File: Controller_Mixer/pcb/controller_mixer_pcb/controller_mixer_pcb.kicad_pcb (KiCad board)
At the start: 2 copper layers, 144.8 x 104.1 mm, 31 parts, among them J1 Conn_01x08_Male, J10 Conn_01x08_Male, J15 Conn_01x05_Male, J16 Conn_01x05_Male, J19 Conn_01x08_Male, J2 Conn_01x08_Male, J20 Conn_01x08_Male, J3 Conn_01x08_Male, J4 Conn_01x08_Male, J5 Conn_01x05_Male, J6 Conn_01x05_Male, J7 Conn_01x08_Male, J8 Conn_01x08_Male, J9 Conn_01x08_Male, U3 Teensy4.1

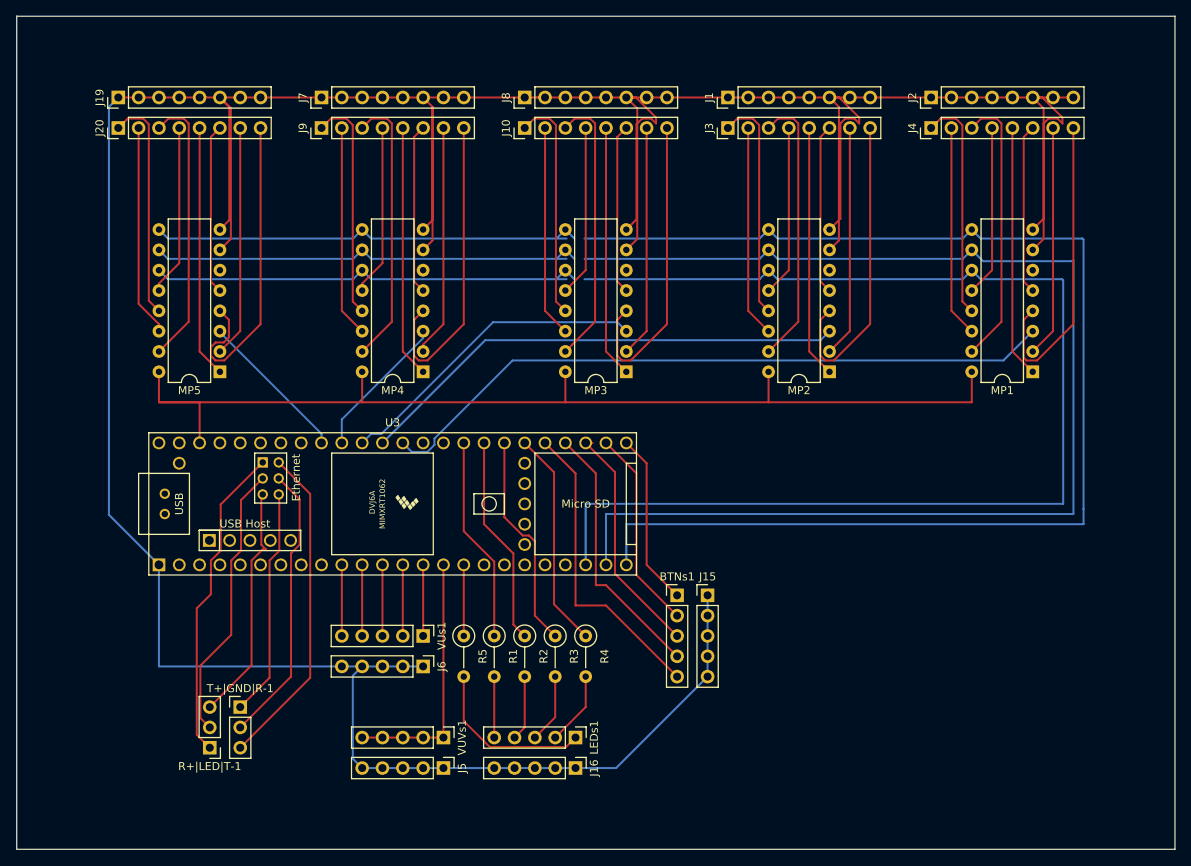
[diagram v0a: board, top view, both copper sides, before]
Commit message: daily edits
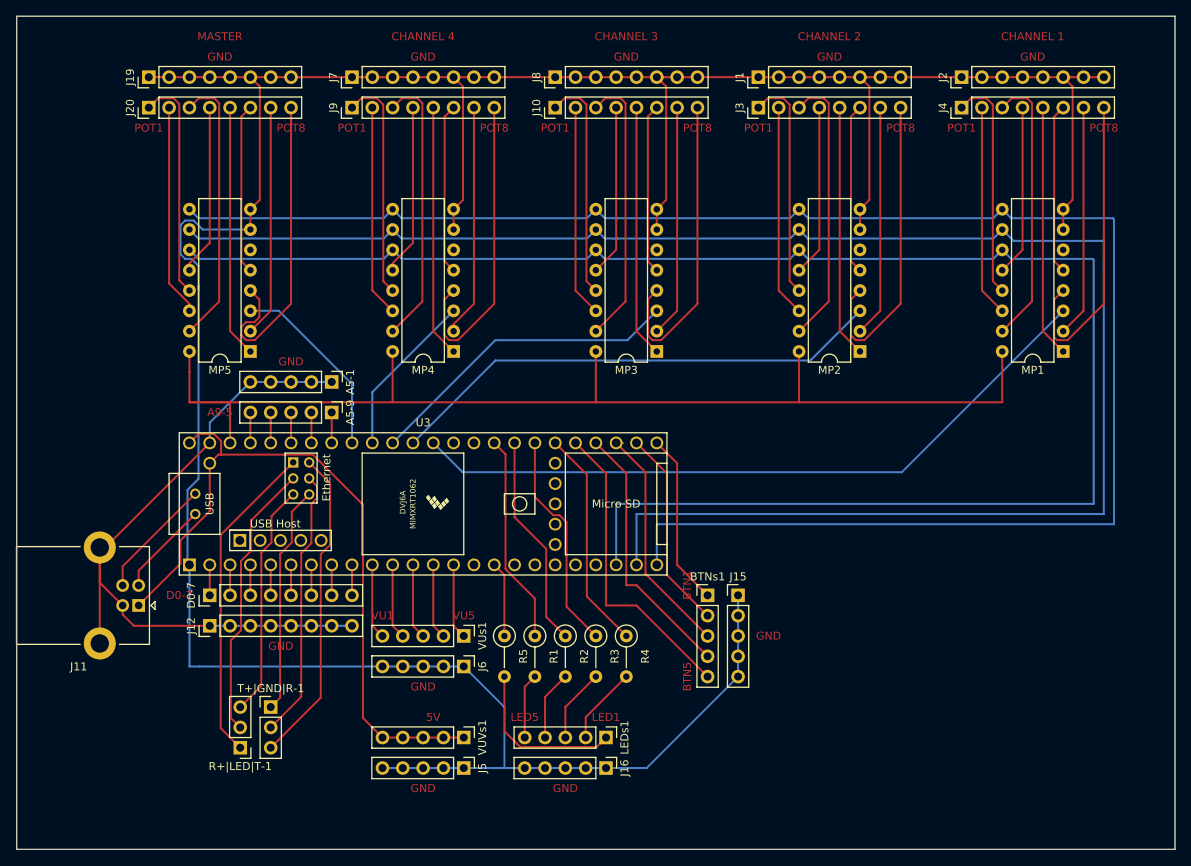
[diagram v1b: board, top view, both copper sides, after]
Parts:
- added A5-1: Conn_01x05_Male, Connector_PinHeader_2.54mm:PinHeader_1x05_P2.54mm_Vertical, F.Cu at (97.8, 85.1)
- added A5-9: Conn_01x05_Male, Connector_PinHeader_2.54mm:PinHeader_1x05_P2.54mm_Vertical, F.Cu at (97.8, 88.9)
- added D0-7: Conn_01x08_Male, Connector_PinHeader_2.54mm:PinHeader_1x08_P2.54mm_Vertical, F.Cu at (82.5, 111.8)
- added J11: USB_B, Connector_USB:USB_B_Lumberg_2411_02_Horizontal, F.Cu at (73.7, 113.0)
- added J12: Conn_01x08_Male, Connector_PinHeader_2.54mm:PinHeader_1x08_P2.54mm_Vertical, F.Cu at (82.5, 115.6)
- moved R4 5.08 mm to (134.6, 116.8)
- moved J6 5.08 mm to (114.3, 120.7)
- moved R1 5.08 mm to (123.2, 116.8)
- moved R2 5.08 mm to (127.0, 116.8)
- moved R3 5.08 mm to (130.8, 116.8)
- moved R5 5.08 mm to (119.4, 116.8)
- moved VUs1 5.08 mm to (114.3, 116.8)
- moved J10 4.58 mm to (125.7, 50.8)
- moved J20 4.58 mm to (74.9, 50.8)
- moved J3 4.58 mm to (151.1, 50.8)
- moved J4 4.58 mm to (176.5, 50.8)
- moved J9 4.58 mm to (100.3, 50.8)
- moved J1 4.58 mm to (151.1, 47.0)
- moved J19 4.58 mm to (74.9, 47.0)
- moved J2 4.58 mm to (176.5, 47.0)
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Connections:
- U3 pad 48: Net-(U3-Pad48) -> Net-(J11-Pad1)
- U3 pad 49: Net-(U3-Pad49) -> Net-(J11-Pad1)
- VUVs1 pad 1: Net-(U3-Pad15) -> Net-(J11-Pad1)
- VUVs1 pad 2: Net-(U3-Pad15) -> Net-(J11-Pad1)
- VUVs1 pad 3: Net-(U3-Pad15) -> Net-(J11-Pad1)
- VUVs1 pad 4: Net-(U3-Pad15) -> Net-(J11-Pad1)
- VUVs1 pad 5: Net-(U3-Pad15) -> Net-(J11-Pad1)
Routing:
- net Net-(J1-Pad1): track 498.8 -> 399.8 mm
- net Net-(J11-Pad1): track 0.00 -> 90.5 mm
- net Net-(A5-1-Pad1): track 0.00 -> 89.9 mm
- net Net-(U3-Pad15): track 31.8 -> 0.00 mm
- net Net-(J11-Pad3): track 0.00 -> 15.2 mm
- net Net-(MP1-Pad16): track 130.8 -> 143.5 mm
- net Net-(J11-Pad2): track 0.00 -> 11.9 mm
- net Net-(MP5-Pad3): track 19.2 -> 24.2 mm
- net Net-(MP1-Pad9): track 217.6 -> 221.7 mm
- net Net-(MP1-Pad10): track 215.2 -> 219.3 mm
- net Net-(D0-7-Pad8): track 0.00 -> 3.81 mm
- net Net-(D0-7-Pad7): track 0.00 -> 3.81 mm
- net Net-(D0-7-Pad6): track 0.00 -> 3.81 mm
- net Net-(D0-7-Pad5): track 0.00 -> 3.81 mm
- net Net-(D0-7-Pad4): track 0.00 -> 3.81 mm
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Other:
- board text added: "5V"
- board text added: "A9-5"
- board text added: "BTN1"
- board text added: "BTN5"
- board text added: "CHANNEL 1"
- board text added: "CHANNEL 2"
- board text added: "CHANNEL 3"
- board text added: "CHANNEL 4"
- board text added: "D0-7"
- board text added: "GND"
- board text added: "LED1"
- board text added: "LED5"
- board text added: "MASTER"
- board text added: "POT1"
- board text added: "POT8"
- board text added: "VU1"
- board text added: "VU5"
